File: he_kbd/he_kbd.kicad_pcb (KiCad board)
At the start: 2 copper layers, 162.2 x 126.5 mm, 175 parts

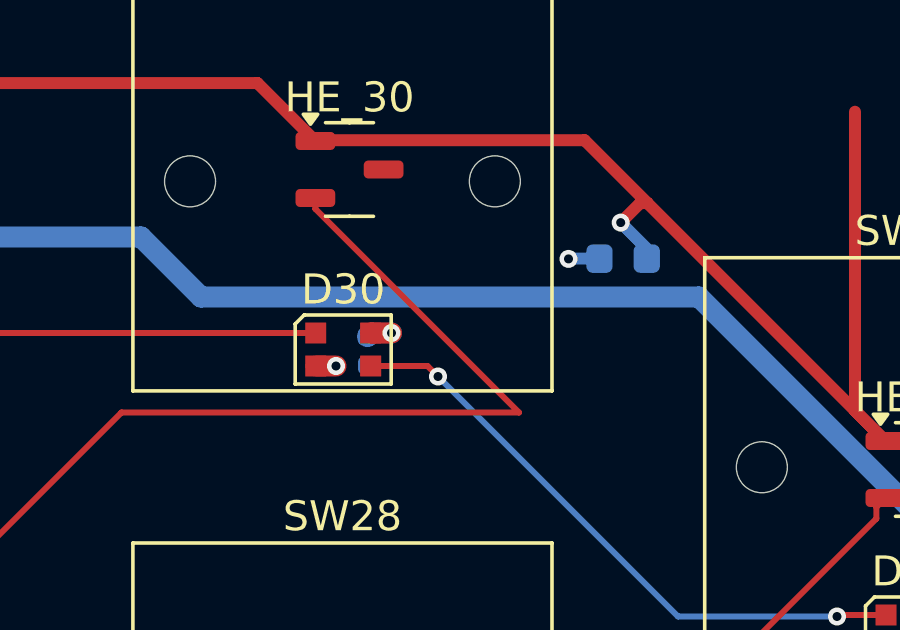
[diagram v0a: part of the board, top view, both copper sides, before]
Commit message: more progress
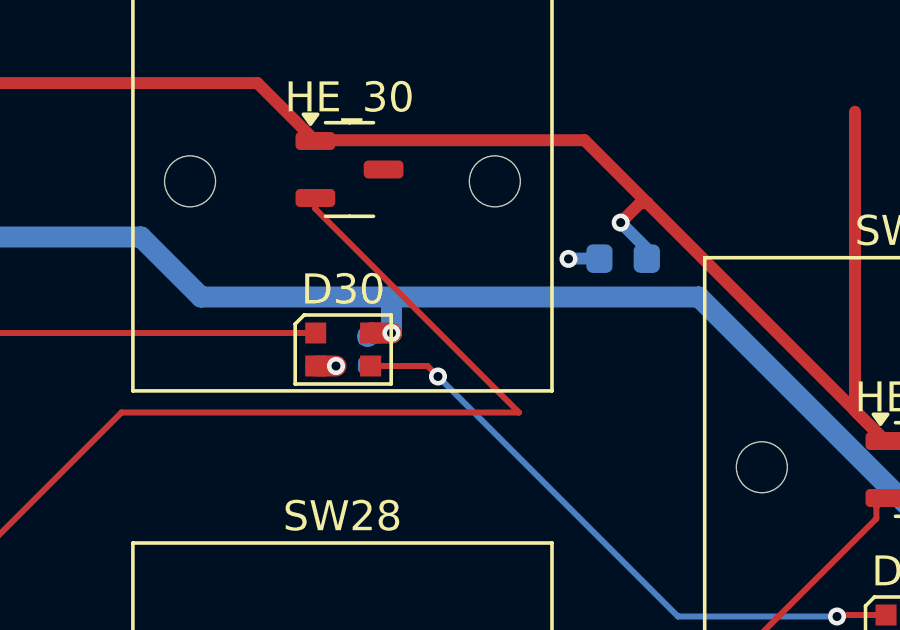
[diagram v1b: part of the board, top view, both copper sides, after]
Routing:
- net NEOPIXEL_POWER: track 914.5 -> 915.7 mm
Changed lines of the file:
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@@
 	)
 	(segment
-		(start 138.240183 50.844942)
+		(start 128.040183 50.844942)
 		(end 121.640183 50.844942)
 		(width 0.7)
@@
 	)
 	(segment
+		(start 138.240183 50.844942)
+		(end 128.040183 50.844942)
+		(width 0.7)
+		(layer "B.Cu")
+		(net 23)
+	)
+	(segment
 		(start 152.460183 85.544942)
 		(end 152.660183 85.344942)
@@
 	)
 	(segment
+		(start 127.990183 50.894942)
+		(end 128.040183 50.844942)
+		(width 0.7)
+		(layer "B.Cu")
+		(net 23)
+	)
+	(segment
 		(start 60.590183 129.094942)
 		(end 59.090183 129.094942)
@@
 		(width 0.7)
 		(layer "B.Cu")
+		(net 23)
+	)
+	(segment
+		(start 127.990183 52.044942)
+		(end 127.990183 50.894942)
+		(width 0.7)
+		(layer "B.Cu")
